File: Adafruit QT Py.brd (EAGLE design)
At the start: 17.8 x 20.7 mm, 27 parts, among them IC3 ATSAMD21E, Q2 reset, U1 AP2112K-3.3, X6 USB TYPE C

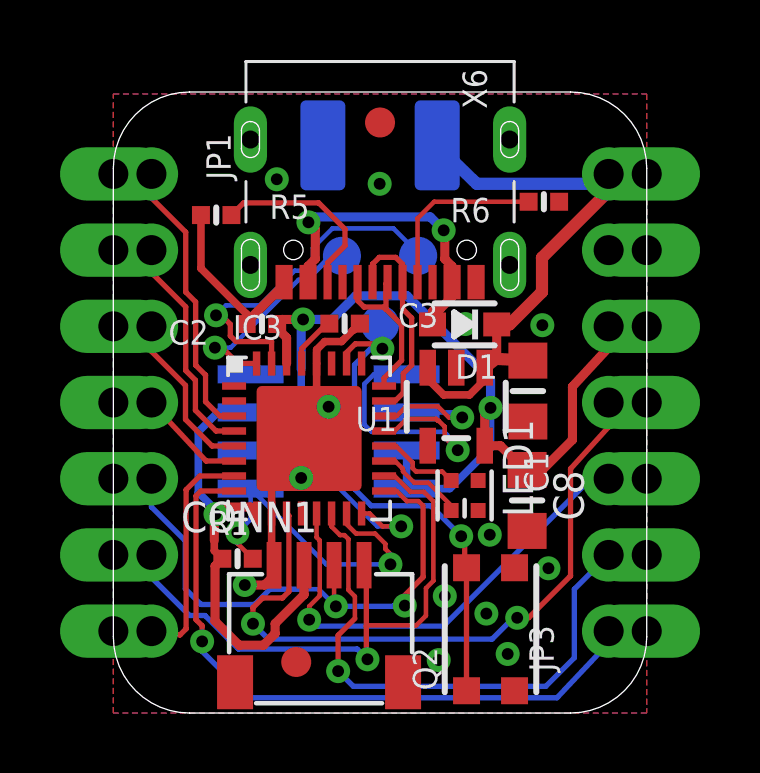
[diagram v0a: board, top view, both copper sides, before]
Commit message: Update board files.
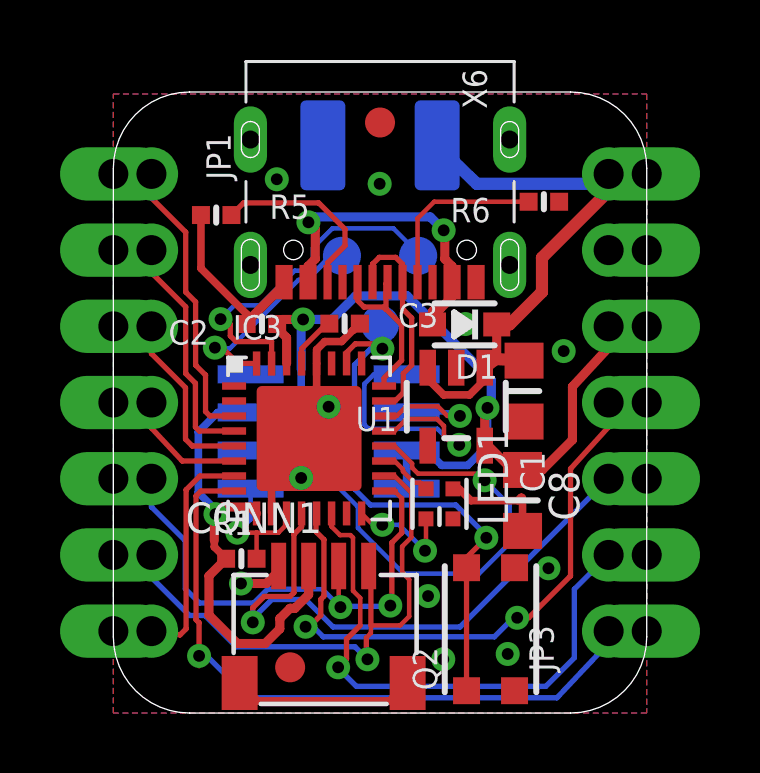
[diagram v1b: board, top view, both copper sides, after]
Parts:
- IC3: device microbuilder:QFN32_5MM -> adafruit_micro:QFN32_5MM
- moved LED1 0.88 mm to (10.9, 6.97)
- moved U$6 0.27 mm to (5.89, 1.52)
- moved CONN1 0.15 mm to (7.01, 2.39)
- moved C8 0.15 mm to (13.6, 7.09)
- moved C1 0.13 mm to (13.7, 10.7)
- moved R1 0.13 mm to (4.27, 5.14)
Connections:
- removed net CS: IC3.15, R1.2, U2.1
- new net FLASH_CS: IC3.11, R1.2, U2.1
- net MISO: now also IC3.12; no longer IC3.13
- net MISO2: now also IC3.20; no longer IC3.16
- net MOSI: now also IC3.13; no longer IC3.11
- net NEOPIX: now also IC3.19; no longer IC3.20
- net NEO_PWR: now also IC3.16; no longer IC3.19
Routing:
- net CS: track 11.1 -> 0.00 mm, vias 2 -> 0
- net MISO2: track 7.57 -> 17.5 mm
- net GND: track 19.9 -> 28.1 mm, vias 13 -> 11
- net FLASH_CS: track 0.00 -> 4.64 mm, vias 0 -> 1
- net MISO: track 17.1 -> 20.8 mm
- net MOSI: track 23.9 -> 21.6 mm
- net SCL: track 21.6 -> 20.5 mm
- net !RESET: track 17.5 -> 18.6 mm
- net SDA: track 19.9 -> 18.8 mm
- net NEOPIX: track 2.82 -> 1.83 mm
- net NEO_PWR: track 3.06 -> 3.72 mm, vias 0 -> 2
- net A3: track 4.96 -> 5.52 mm
